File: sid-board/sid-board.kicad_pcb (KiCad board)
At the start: 2 copper layers, 13 parts, among them J1 ICM_CONN, J2 SID_CONN, J3 5V/GND, J4 3.3V/GND, J5 SPI, J6 UARTAB/IRQ, U1 SC16IS752IPW, U2 LM2596MODULE, U3 PCA82C250, U4 PCA82C250

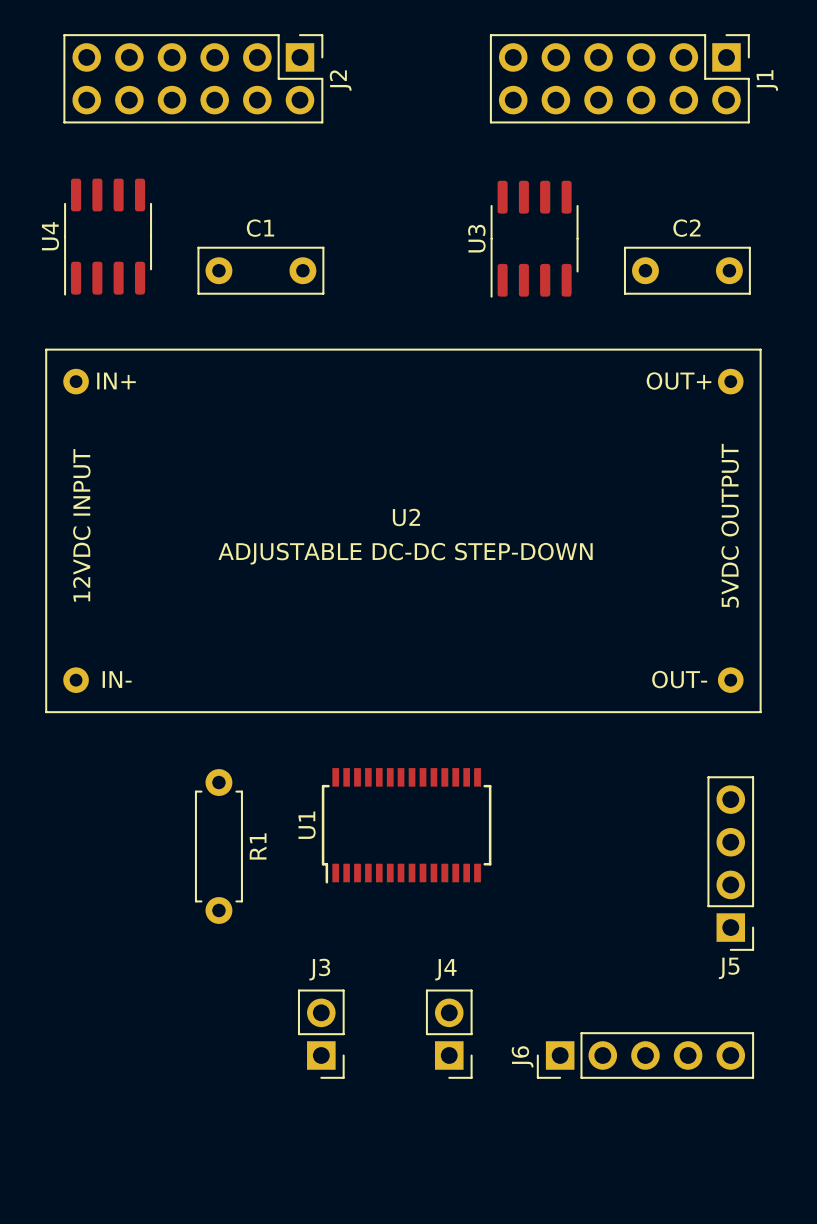
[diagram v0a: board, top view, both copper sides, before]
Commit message: Happy with first prototype, going to try get it made!
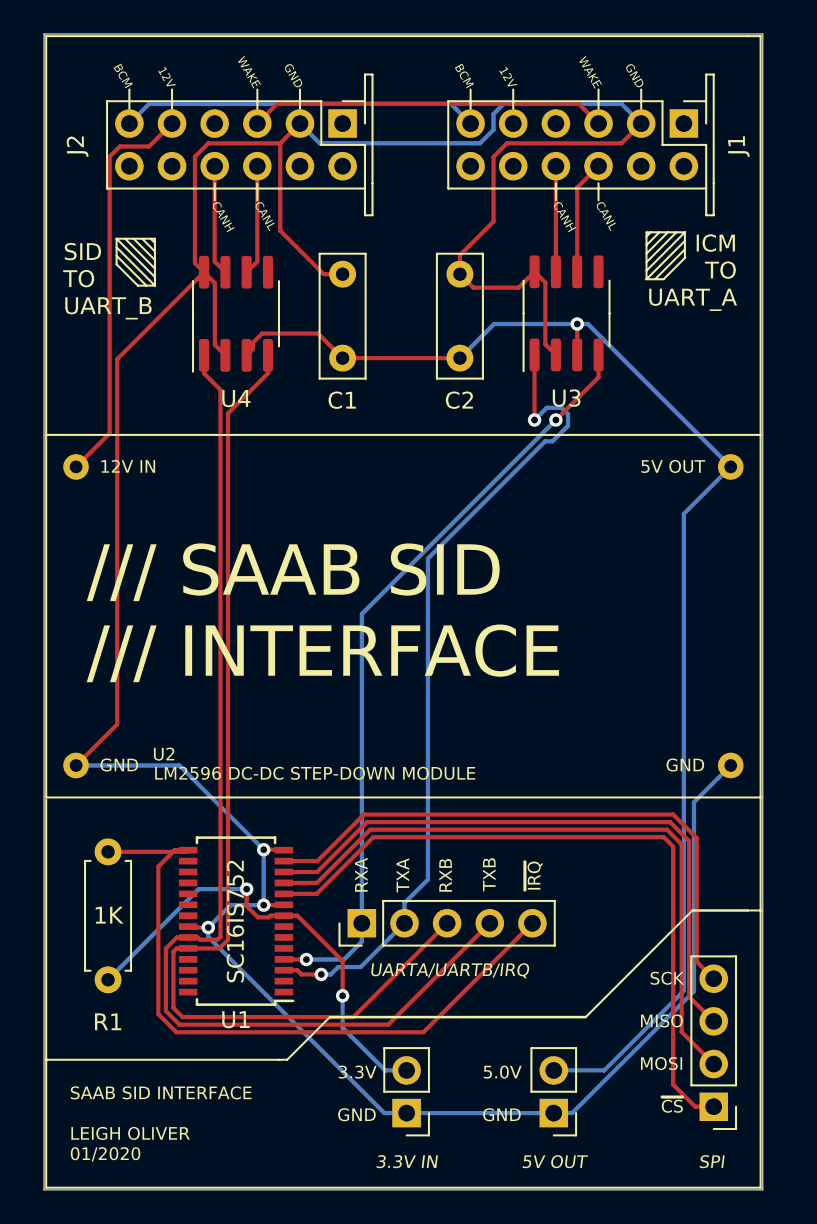
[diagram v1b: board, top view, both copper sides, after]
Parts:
- J1, J2: footprint Connector_PinHeader_2.54mm:PinHeader_2x06_P2.54mm_Vertical -> sid-board:SAAB_SID_CONNECTOR_HEADER
- J3: value 5V/GND -> 5V OUT
- J4: value 3.3V/GND -> 3.3V IN
- J6: value UARTAB/IRQ -> UARTA/UARTB/IRQ
- U1: value SC16IS752IPW -> SC16IS752
- moved J3 14.3 mm to (92.6, 123.8)
- moved J6 14.2 mm to (81.2, 112.5)
- moved C2 12.2 mm to (87.0, 78.9), turned to 90 degrees
- moved U1 11.7 mm to (73.7, 112.4), turned to 180 degrees
- moved SPI 10.7 mm to (102.1, 123.4)
- moved J1 10.2 mm to (94.0, 66.0), turned to 0 degrees
- moved C1 9.02 mm to (80.0, 78.9), turned to 90 degrees
- moved U4 8.90 mm to (73.7, 76.2)
- moved R1 7.79 mm to (66.0, 108.3)
- moved J2 6.35 mm to (73.7, 66.0), turned to 0 degrees
- moved U2 5.08 mm to (83.8, 94.0)
- moved U3 4.84 mm to (93.3, 76.2)
- moved J4 4.27 mm to (83.8, 123.8)
- renumbered J5 to SPI
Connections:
- U3 pad 4: (no net) -> Net-(J6-Pad1)
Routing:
- net GND: track 0.00 -> 188.3 mm, vias 0 -> 3
- net VDD_5V: track 0.00 -> 78.5 mm, vias 0 -> 1
- net Net-(J6-Pad4): track 0.00 -> 64.5 mm
- net Net-(J6-Pad3): track 0.00 -> 61.5 mm
- net Net-(J6-Pad2): track 0.00 -> 49.5 mm, vias 0 -> 2
- net Net-(J6-Pad1): track 0.00 -> 45.9 mm, vias 0 -> 2
- net Net-(J5-Pad1): track 0.00 -> 41.9 mm
- net Net-(J6-Pad5): track 0.00 -> 41.2 mm
- net Net-(J5-Pad2): track 0.00 -> 39.2 mm
- net Net-(J5-Pad3): track 0.00 -> 37.2 mm
- net Net-(J5-Pad4): track 0.00 -> 35.1 mm
- net VDD_3.3V: track 0.00 -> 27.5 mm, vias 0 -> 2
- net VIN: track 0.00 -> 23.8 mm
- net Net-(J1-Pad6): track 0.00 -> 21.3 mm
- net Net-(J1-Pad3): track 0.00 -> 21.3 mm
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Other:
- board outline added: 42.8 x 68.8 mm
- board text added: "/// DESCRIPTION Provides an SPI breakout to a DUAL-UART interface, allowing for REVERSE-ENGINEERING of the SAAB SID/HPD. Designed for SAAB 9-3 Second Generation models (2003+), with high position SID. /// APPLICATION 1. Unplug SID. 2. Plug SID cable into ICM port (J1). 3. Connect SID to SID port (J2) via appropriate 12-core cable. 4. Interface to SPI bus with appropriate microcontroller."
- board text added: "/// SAAB SID /// INTERFACE"
- board text added: "3.3V"
- board text added: "5.0V"
- board text added: "GND"
- board text added: "ICM TO UART_A"
- board text added: "MISO"
- board text added: "MOSI"
- board text added: "RXA"
- board text added: "RXB"
- board text added: "SAAB SID INTERFACE LEIGH OLIVER 01/2020"
- board text added: "SCK"
- board text added: "SID TO UART_B"
- board text added: "TXA"
- board text added: "TXB"
- board text added: "~CS"
- board text added: "~IRQ"
